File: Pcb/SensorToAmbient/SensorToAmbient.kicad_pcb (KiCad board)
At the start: 2 copper layers, 48.1 x 69.7 mm, 17 parts, among them J1 Conn_01x04, J2 Conn_01x04, J3 Conn_01x04, J4 Conn_01x04, J5 Conn_01x04, J6 Conn_01x04, J7 Conn_01x02, J8 Conn_01x06, J9 Conn_01x06

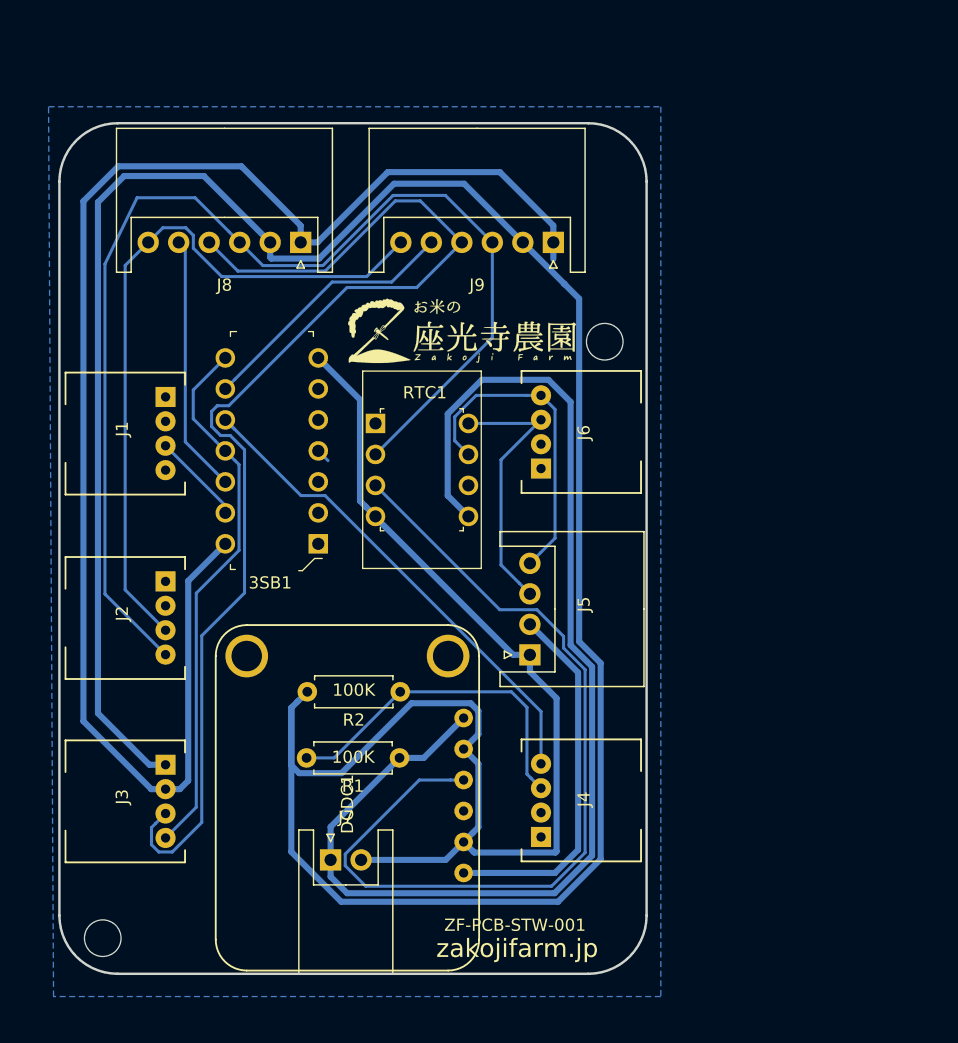
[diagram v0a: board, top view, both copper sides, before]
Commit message: Commit intermediate (Making double-side board)
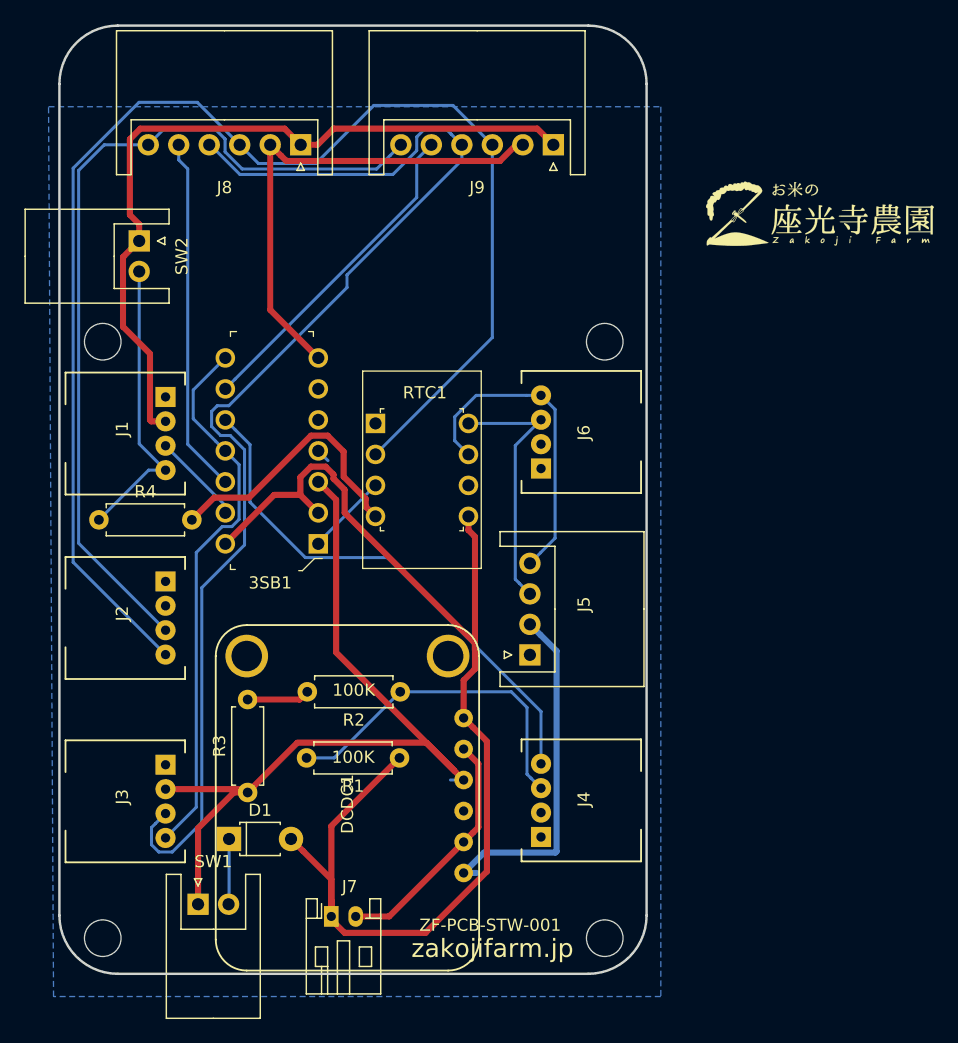
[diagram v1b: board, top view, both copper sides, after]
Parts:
- added D1: D_Schottky, Diodes_THT:D_T-1_P5.08mm_Horizontal, F.Cu at (36.6, 76.5)
- added R3: R, Resistors_THT:R_Axial_DIN0207_L6.3mm_D2.5mm_P7.62mm_Horizontal, F.Cu at (38.1, 72.6)
- added R4: R, Resistors_THT:R_Axial_DIN0207_L6.3mm_D2.5mm_P7.62mm_Horizontal, F.Cu at (25.9, 50.3)
- added REF**: MountingHole_3mm_rev, SensorToAmbient:MountingHole_3mm_rev, F.Cu at (67.4, 84.6)
- added REF**: MountingHole_3mm_rev, SensorToAmbient:MountingHole_3mm_rev, F.Cu at (26.2, 35.7)
- added SW1: SW_Push, Connectors_JST:JST_XH_S02B-XH-A_02x2.50mm_Angled, F.Cu at (34.0, 81.8)
- added SW2: SW_Push, Connectors_JST:JST_XH_S02B-XH-A_02x2.50mm_Angled, F.Cu at (29.2, 27.4)
- J7: footprint Connectors_JST:JST_XH_S02B-XH-A_02x2.50mm_Angled -> Connectors_JST:JST_PH_S2B-PH-K_02x2.00mm_Angled
- moved G*** 30.9 mm to (85.3, 25.1)
- moved J8 8.00 mm to (42.5, 19.6)
- moved J9 8.00 mm to (63.2, 19.6)
- moved J7 4.63 mm to (45.0, 82.8)
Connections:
- 3SB1 pad 14: /PWR3.3V -> /PWR_BAT
- 3SB1 pad 2: Net-(3SB1-Pad2) -> /PWR_BAT
- 3SB1 pad 3: Net-(3SB1-Pad3) -> /PWR3.3V
- DCDC1 pad 3: Net-(DCDC1-Pad3) -> /PWR3.3V
- J1 pad 2: Net-(J1-Pad2) -> /PWR3.3V
- RTC1 pad 3: Net-(DCDC1-Pad3) -> Net-(3SB1-Pad1)
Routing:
- net GND: track 290.1 -> 88.4 mm
- net Net-(DCDC1-Pad3): track 73.7 -> 0.00 mm
- net Net-(J1-Pad4): track 0.00 -> 24.3 mm
- net Net-(J2-Pad4): track 96.9 -> 114.3 mm
- net Net-(J2-Pad3): track 58.6 -> 71.2 mm
- net Net-(3SB1-Pad12): track 21.2 -> 29.2 mm
- net Net-(3SB1-Pad1): track 0.00 -> 6.73 mm
- net /PWR3.3V: track 124.5 -> 131.2 mm
- net Net-(D1-Pad1): track 0.00 -> 5.37 mm
- net Net-(3SB1-Pad9): track 21.9 -> 27.0 mm
- net Net-(J3-Pad3): track 96.9 -> 100.4 mm
- net /PWR_BAT: track 101.0 -> 104.3 mm
- net Net-(3SB1-Pad10): track 41.2 -> 42.8 mm
- net /PWR5V: track 30.3 -> 28.9 mm
- net Net-(J5-Pad3): track 22.7 -> 21.7 mm
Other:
- board size 48.1 x 69.7 mm -> 48.1 x 77.7 mm
